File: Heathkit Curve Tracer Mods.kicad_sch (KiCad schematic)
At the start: 13 parts, among them J1 Switch, J2 IC6 Jumper, J3 +15, U1 74LS42, U2 74LVC1G04, U3 74LS90, U4 LM7805_TO220

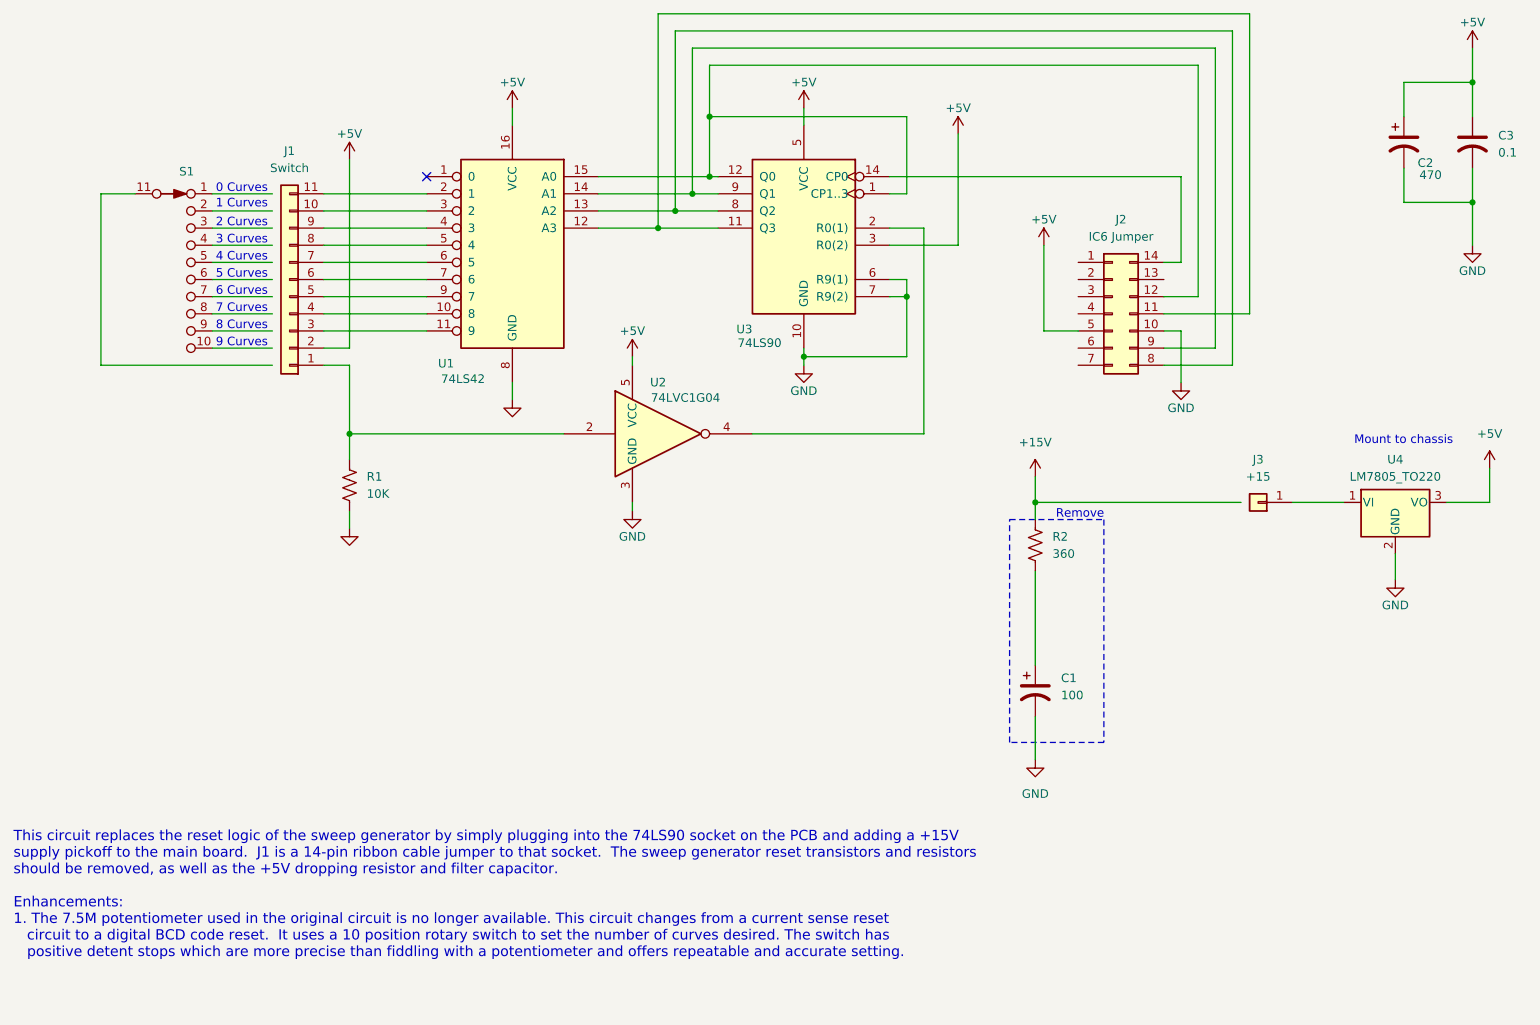
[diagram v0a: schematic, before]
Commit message: updates
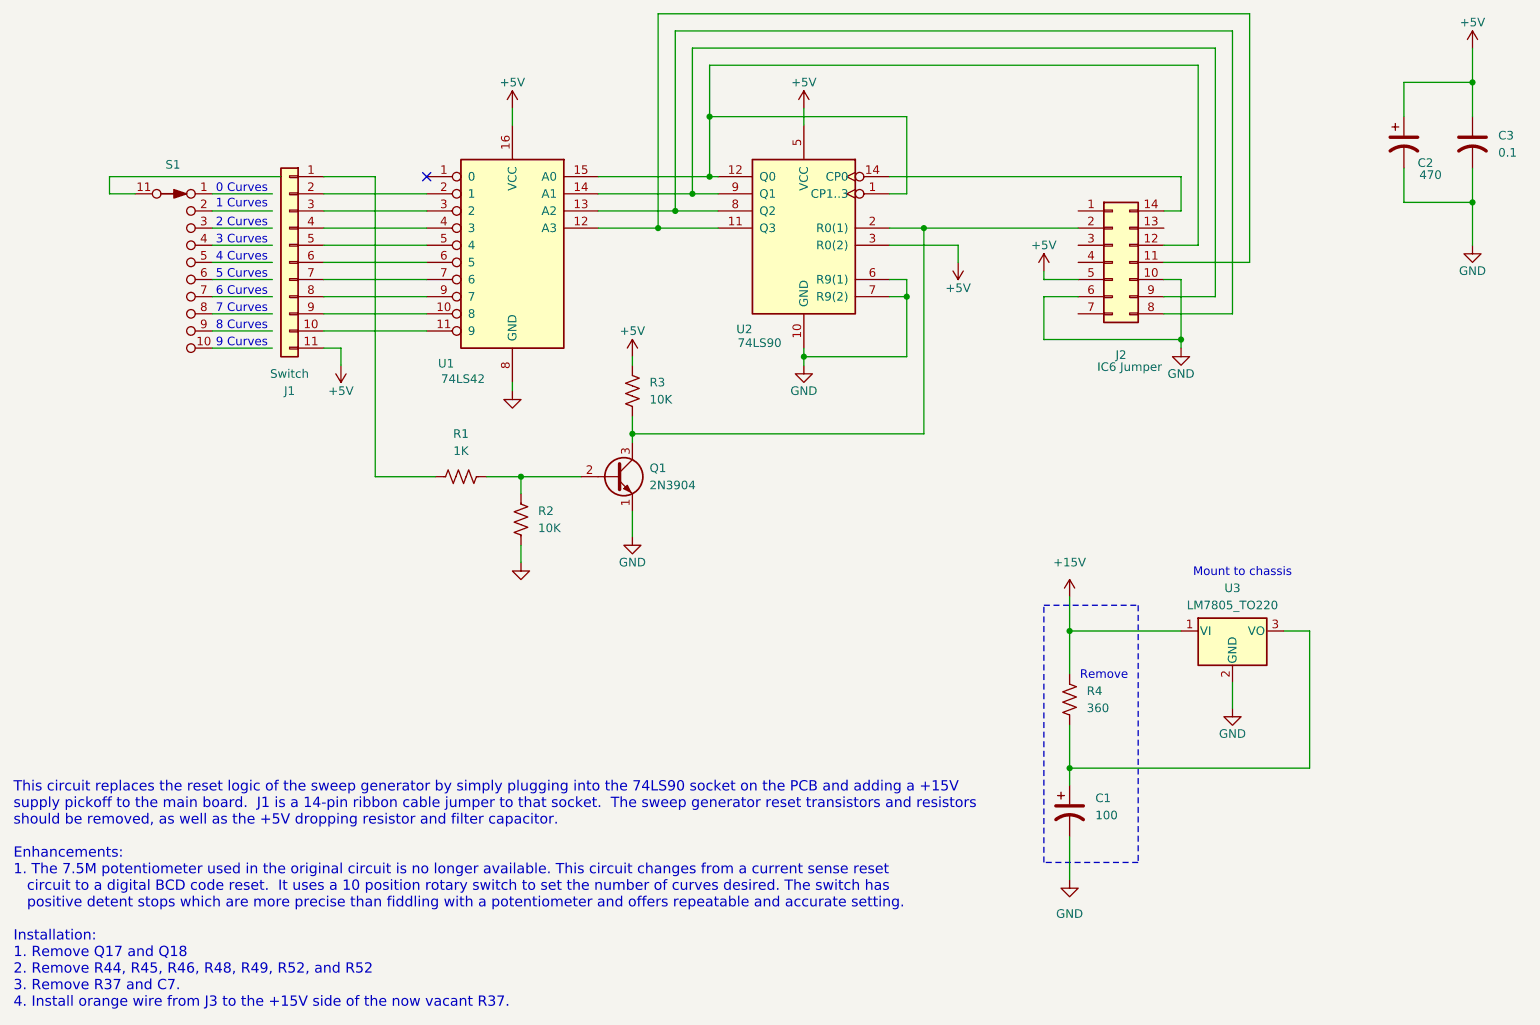
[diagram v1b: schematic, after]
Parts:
- removed J3: +15, Connector_Pin:Pin_D1.3mm_L11.0mm_LooseFit, symbol Connector_Generic:Conn_01x01
- removed U2: 74LVC1G04, Package_TO_SOT_SMD:SOT-23-5, symbol 74xGxx:74LVC1G04
- added Q1: 2N3904, Package_TO_SOT_THT:TO-92L_HandSolder, symbol Transistor_BJT:2N3904
- added R1: 1K, Resistor_THT:R_Axial_DIN0207_L6.3mm_D2.5mm_P7.62mm_Horizontal, symbol Device:R_US
- added R3: 10K, Resistor_THT:R_Axial_DIN0207_L6.3mm_D2.5mm_P7.62mm_Horizontal, symbol Device:R_US
- C2: footprint Capacitor_SMD:CP_Elec_10x14.3 -> Capacitor_THT:CP_Radial_D10.0mm_P3.80mm
- C3: footprint Capacitor_SMD:C_0805_2012Metric_Pad1.18x1.45mm_HandSolder -> Capacitor_THT:C_Disc_D4.7mm_W2.5mm_P5.00mm
- J2: footprint Package_DIP:DIP-14_W7.62mm_LongPads -> Package_DIP:DIP-14_W7.62mm_Socket_LongPads
- R2: renamed from R1; footprint Resistor_SMD:R_0805_2012Metric_Pad1.20x1.40mm_HandSolder -> Resistor_THT:R_Axial_DIN0207_L6.3mm_D2.5mm_P7.62mm_Horizontal
- U1: footprint Package_SO:SOIC-16W_5.3x10.2mm_P1.27mm -> Package_DIP:DIP-16_W7.62mm_Socket_LongPads
- U2: renamed from U3; footprint Package_SO:SOIC-14_3.9x8.7mm_P1.27mm -> Package_DIP:DIP-14_W7.62mm_Socket_LongPads
- renumbered R2 to R4, U4 to U3
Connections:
- net +15V: now also U3.1 (VI)
- net +5V: now also J1.11 (Pin_11), R3.1; no longer J1.2 (Pin_2), U3.3 (VO)
- net GND: now also J2.6 (Pin_6), Q1.1 (E)
- net at J2.2 (Pin_2): now also U2.2 (R0(1)), Q1.3 (C), R3.2
- net at C1.1, R4.2: now also U3.3 (VO)
- net at U1.10 (8): now also J1.9 (Pin_9); no longer J1.4 (Pin_4)
- net at U1.11 (9): now also J1.10 (Pin_10); no longer J1.3 (Pin_3)
- net at U1.2 (1): now also J1.2 (Pin_2); no longer J1.11 (Pin_11)
- net at U1.3 (2): now also J1.3 (Pin_3); no longer J1.10 (Pin_10)
- net at U1.4 (3): now also J1.4 (Pin_4); no longer J1.9 (Pin_9)
- net at U1.5 (4): now also J1.5 (Pin_5); no longer J1.8 (Pin_8)
- net at U1.6 (5): now also J1.6 (Pin_6); no longer J1.7 (Pin_7)
- net at U1.7 (6): now also J1.7 (Pin_7); no longer J1.6 (Pin_6)
- net at U1.9 (7): now also J1.8 (Pin_8); no longer J1.5 (Pin_5)
- net at R2.1: now also Q1.2 (B), R1.2; no longer J1.1 (Pin_1)
- new net: J1.1 (Pin_1), R1.1
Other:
- moved on the sheet: C1, J1, J2, R2, R4, U3
